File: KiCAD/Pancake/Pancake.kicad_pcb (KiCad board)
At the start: 2 copper layers, 191 parts, among them IC10 LF347N, IC3 LF347N, IC4 LF347N, IC5 LF347N, IC6 LF347N, IC7 LF347N, IC8 LF347N, IC9 LF347N, J1 Conn_01x08_Male, J101 TB001-500-04BE, J102 TB001-500-03BE, J2 Conn_01x08_Male, J3 Conn_01x08_Male, J4 Conn_01x08_Male, J5 Conn_01x08_Male, J7 Conn_02x15_Top_Bottom, Q901 ULN2003AIN, Q902 ULN2003AIN

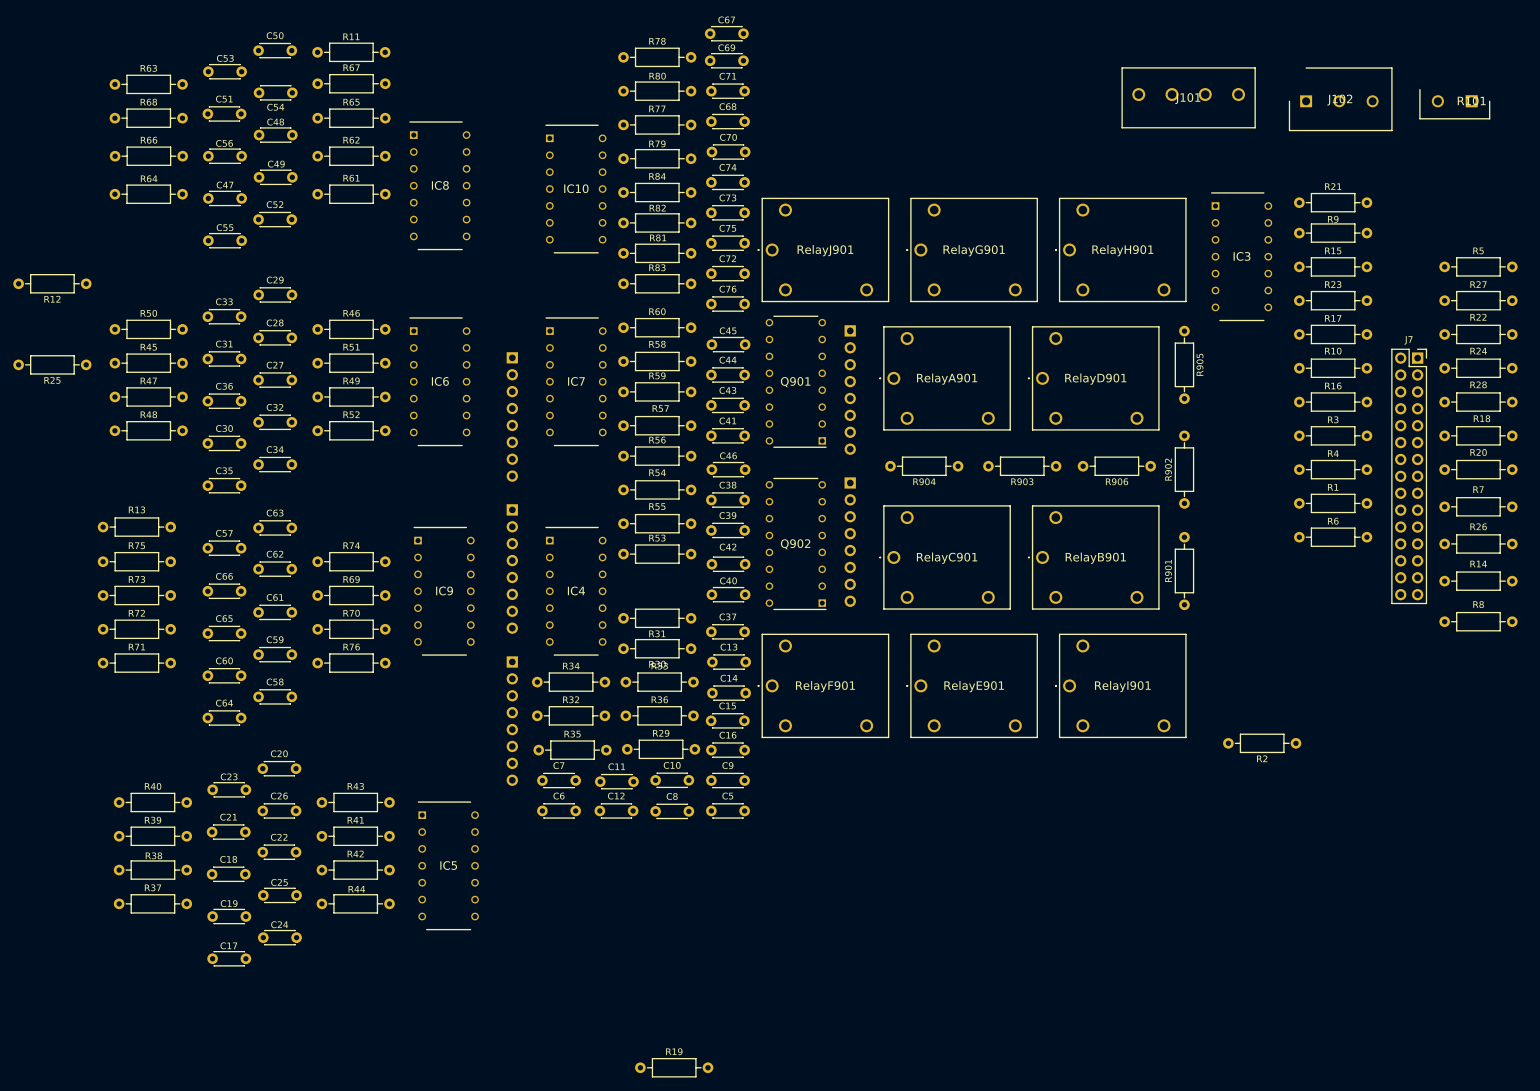
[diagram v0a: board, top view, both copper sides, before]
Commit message: Latest revision
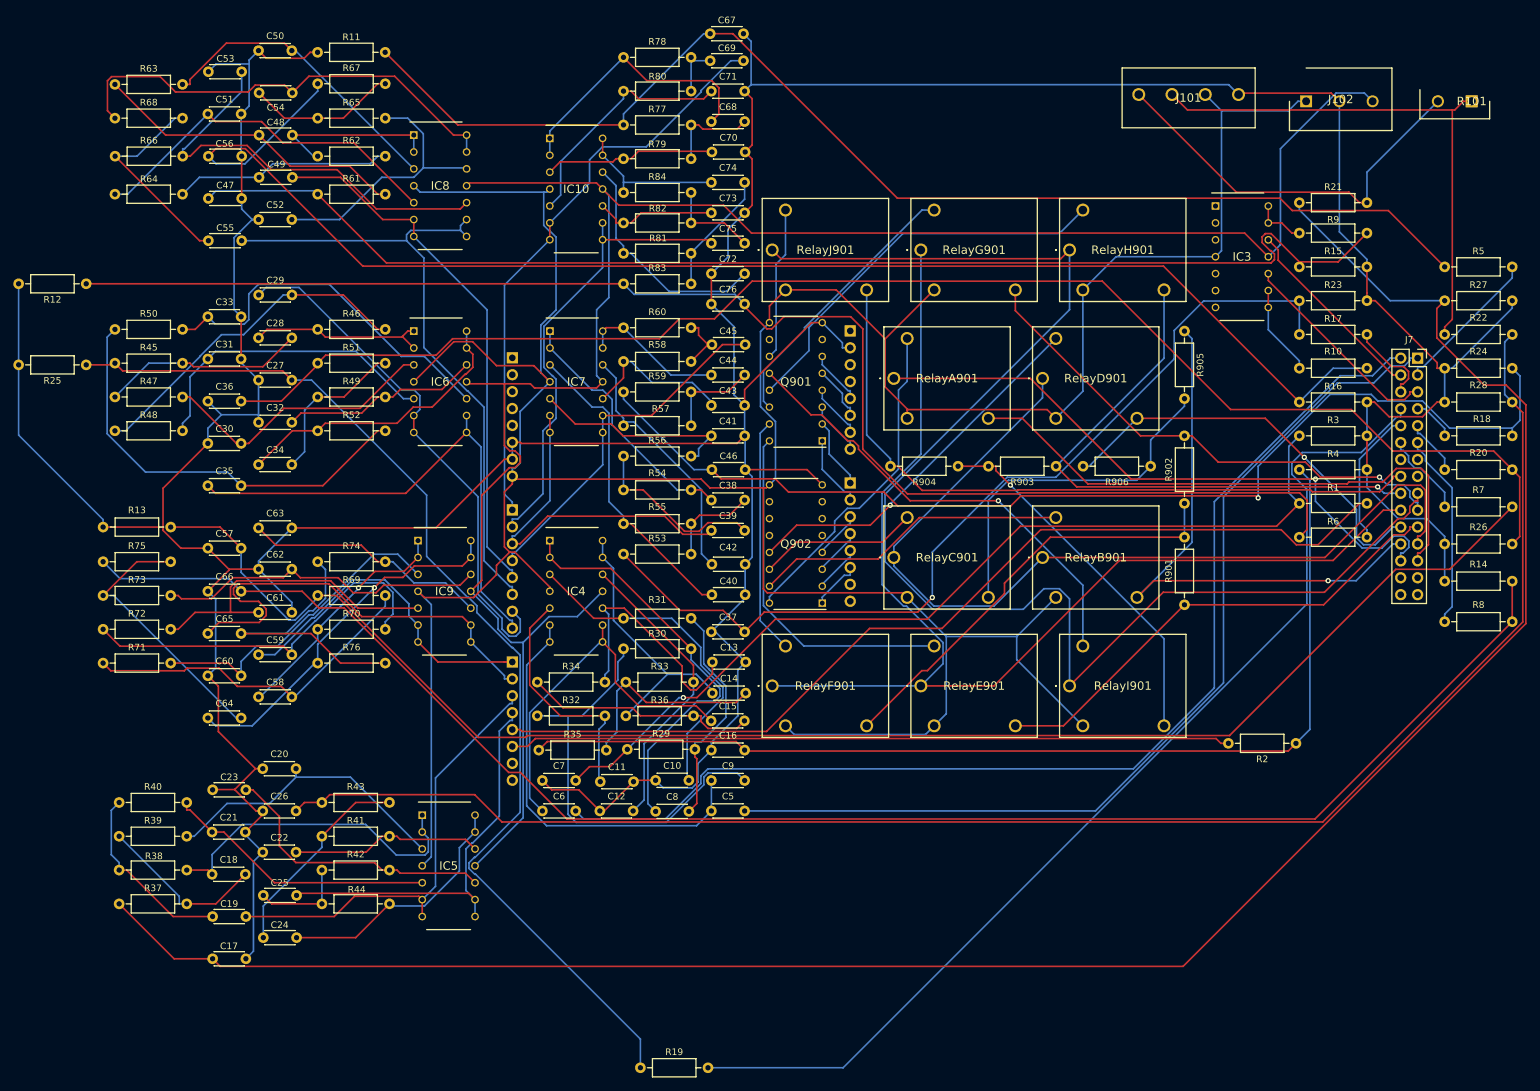
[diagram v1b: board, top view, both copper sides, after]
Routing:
- net GND: track 0.00 -> 740.3 mm
- net +12V: track 0.00 -> 513.6 mm
- net /ADC1011/IN1: track 0.00 -> 321.8 mm
- net -12V: track 0.00 -> 311.8 mm
- net /ADC89/IN2: track 0.00 -> 246.2 mm
- net /ADC1011/IN2: track 0.00 -> 244.4 mm
- net /ADC89/IN1: track 0.00 -> 234.5 mm
- net /ADC67/IN2: track 0.00 -> 222.5 mm
- net /ADC01/IN2: track 0.00 -> 215.5 mm
- net /DriveMid: track 0.00 -> 215.4 mm
- net /ADC45/IN2: track 0.00 -> 215.1 mm
- net /ADC45/IN1: track 0.00 -> 190.0 mm
- net /ADC01/IN1: track 0.00 -> 185.0 mm
- net /ToneMid: track 0.00 -> 178.8 mm
- net /AuxIn: track 0.00 -> 170.3 mm
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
